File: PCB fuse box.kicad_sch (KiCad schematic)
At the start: 22 parts, among them J1 6570XX230201_657012230201, J2 6570XX230201_657012230201, J3 449140201, J4 449140201, K1 AZ2150-1A-12DEF, K2 AZ2150-1A-12DEF

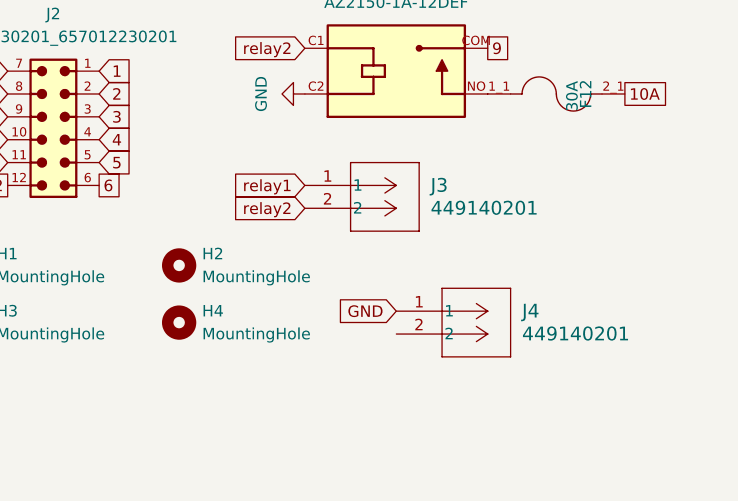
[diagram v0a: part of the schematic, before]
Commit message: fix smth
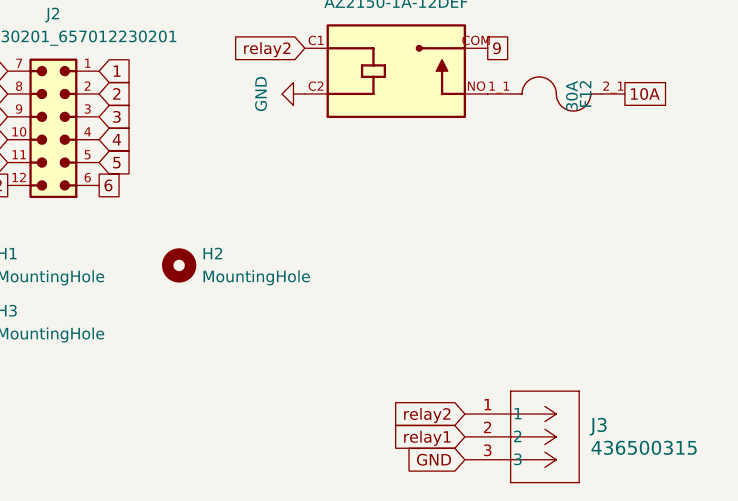
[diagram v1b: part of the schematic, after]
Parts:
- removed H4: MountingHole, MountingHole:MountingHole_2.2mm_M2_Pad, symbol Mechanical:MountingHole
- removed J3, J4: 449140201, fuse-relay_NewFootprints:CONN_SD-44914-002_02_MOL, symbol New_Library:449140201
- added J3: 436500315, MOLEX 436500315:CONN_SD-43650-006_03_MOL, symbol MOLEX 436500315:436500315
- F1, F10, F11, F12, F2, F3, F4, F5, F6, F7, F8, F9: footprint fuse-relay_NewFootprints:FUSE_3557-2 -> 3557:CONN_3557-2_KEY
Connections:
- net GND: now also J3.3
- net relay1: now also J3.2
- net relay2: now also J3.1
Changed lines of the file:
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@@
 	(global_label "relay1"
 		(shape input)
-		(at 104.14 77.47 180)
+		(at 121.92 105.41 180)
 		(fields_autoplaced yes)
 		(effects
@@
 		)
 		(property "Intersheetrefs" "${INTERSHEET_REFS}"
-			(at 95.2887 77.47 0)
+			(at 113.0687 105.41 0)
 			(hide yes)
 			(show_name no)
@@
 	(global_label "relay2"
 		(shape input)
-		(at 104.14 80.01 180)
+		(at 121.92 102.87 180)
 		(fields_autoplaced yes)
 		(effects
@@
 		)
 		(property "Intersheetrefs" "${INTERSHEET_REFS}"
-			(at 95.2887 80.01 0)
+			(at 113.0687 102.87 0)
 			(hide yes)
 			(show_name no)
@@
 	(global_label "GND"
 		(shape input)
-		(at 114.3 91.44 180)
+		(at 121.92 107.95 180)
 		(fields_autoplaced yes)
 		(effects
@@
 		)
 		(property "Intersheetrefs" "${INTERSHEET_REFS}"
-			(at 107.4443 91.44 0)
+			(at 115.0643 107.95 0)
 			(hide yes)
 			(show_name no)
@@
 	)
 	(symbol
+		(lib_id "MOLEX 436500315:436500315")
+		(at 121.92 102.87 0)
+		(unit 1)
+		(body_style 1)
+		(exclude_from_sim no)
+		(in_bom yes)
+		(on_board yes)
+		(in_pos_files yes)
+		(dnp no)
+		(fields_autoplaced yes)
+		(property "Reference" "J3"
+			(at 135.89 104.1399 0)
+			(show_name no)
+			(do_not_autoplace no)
+			(effects
+				(font
+					(size 1.524 1.524)
+				)
+				(justify left)
+			)
+		)
+		(property "Value" "436500315"
+			(at 135.89 106.6799 0)
+			(show_name no)
+			(do_not_autoplace no)
+			(effects
+				(font
+					(size 1.524 1.524)
+				)
+				(justify left)
+			)
+		)
+		(property "Footprint" "MOLEX 436500315:CONN_SD-43650-006_03_MOL"
+			(at 121.92 102.87 0)
+			(hide yes)
+			(show_name no)
+			(do_not_autoplace no)
+			(effects
+				(font
+					(size 1.27 1.27)
+					(italic yes)
+				)
+			)
+		)
+		(property "Datasheet" "https://www.molex.com/en-us/products/part-detail-pdf/436500315?display=pdf"
+			(at 121.92 102.87 0)
+			(hide yes)
+			(show_name no)
+			(do_not_autoplace no)
+			(effects
+				(font
+					(size 1.27 1.27)
+					(italic yes)
+				)
+			)
+		)
+		(property "Description" ""
+			(at 121.92 102.87 0)
+			(hide yes)
+			(show_name no)
+			(do_not_autoplace no)
+			(effects
+				(font
+					(size 1.27 1.27)
+				)
+			)
+		)
+		(pin "3"
+		)
+		(pin "1"
+		)
+		(pin "2"
+		)
+		(instances
+			(project "PCB fuse box"
+				(path "/edb1809c-767d-4732-82a5-e09154bd7612"
+					(reference "J3")
+					(unit 1)
+				)
+			)
+		)
+	)
+	(symbol
 		(lib_id "New_Library:3557-2")
 		(at 25.4 68.58 270)
@@
 			)
 		)
-		(property "Footprint" "fuse-relay_NewFootprints:FUSE_3557-2"
+		(property "Footprint" "3557:CONN_3557-2_KEY"
 			(at 25.4 68.58 0)
 			(hide yes)
@@
 			)
 		)
-		(property "Footprint" "fuse-relay_NewFootprints:FUSE_3557-2"
+		(property "Footprint" "3557:CONN_3557-2_KEY"
 			(at 35.56 41.91 0)
 			(hide yes)
@@
 			)
 		)
-		(property "Footprint" "fuse-relay_NewFootprints:FUSE_3557-2"
+		(property "Footprint" "3557:CONN_3557-2_KEY"
 			(at 55.88 68.58 0)
 			(hide yes)
@@
 	)
 	(symbol
-		(lib_id "Mechanical:MountingHole")
-		(at 90.17 92.71 0)
-		(unit 1)
-		(body_style 1)
-		(exclude_from_sim no)
-		(in_bom no)
-		(on_board yes)
-		(in_pos_files yes)
-		(dnp no)
-		(fields_autoplaced yes)
-		(property "Reference" "H4"
-			(at 92.71 91.4399 0)
-			(show_name no)
-			(do_not_autoplace no)
-			(effects
-				(font
-					(size 1.27 1.27)
-				)
-				(justify left)
-			)
-		)
-		(property "Value" "MountingHole"
-			(at 92.71 93.9799 0)
-			(show_name no)
-			(do_not_autoplace no)
-			(effects
-				(font
-					(size 1.27 1.27)
-				)
-				(justify left)
-			)
-		)
-		(property "Footprint" "MountingHole:MountingHole_2.2mm_M2_Pad"
-			(at 90.17 92.71 0)
-			(hide yes)
-			(show_name no)
-			(do_not_autoplace no)
-			(effects
-				(font
-					(size 1.27 1.27)
-				)
-			)
-		)
-		(property "Datasheet" ""
-			(at 90.17 92.71 0)
-			(hide yes)
-			(show_name no)
-			(do_not_autoplace no)
-			(effects
-				(font
-					(size 1.27 1.27)
-				)
-			)
-		)
-		(property "Description" "Mounting Hole without connection"
-			(at 90.17 92.71 0)
-			(hide yes)
-			(show_name no)
-			(do_not_autoplace no)
-			(effects
-				(font
-					(size 1.27 1.27)
-				)
-			)
-		)
-		(instances
-			(project "PCB fuse box"
-				(path "/edb1809c-767d-4732-82a5-e09154bd7612"
-					(reference "H4")
-					(unit 1)
-				)
-			)
-		)
-	)
-	(symbol
 		(lib_id "New_Library:3557-2")
 		(at 36.83 93.98 270)
@@
 			)
 		)
-		(property "Footprint" "fuse-relay_NewFootprints:FUSE_3557-2"
+		(property "Footprint" "3557:CONN_3557-2_KEY"
 			(at 36.83 93.98 0)
 			(hide yes)
@@
 			)
 		)
-		(property "Footprint" "fuse-relay_NewFootprints:FUSE_3557-2"
+		(property "Footprint" "3557:CONN_3557-2_KEY"
 			(at 132.08 41.91 0)
 			(hide yes)
@@
 			)
 		)
-		(property "Footprint" "fuse-relay_NewFootprints:FUSE_3557-2"
+		(property "Footprint" "3557:CONN_3557-2_KEY"
 			(at 35.56 68.58 0)
 			(hide yes)
@@
 	)
 	(symbol
-		(lib_id "New_Library:449140201")
-		(at 114.3 91.44 0)
-		(unit 1)
-		(body_style 1)
-		(exclude_from_sim no)
-		(in_bom yes)
-		(on_board yes)
-		(in_pos_files yes)
-		(dnp no)
-		(fields_autoplaced yes)
-		(property "Reference" "J4"
-			(at 128.27 91.4399 0)
-			(show_name no)
-			(do_not_autoplace no)
-			(effects
-				(font
-					(size 1.524 1.524)
-				)
-				(justify left)
-			)
-		)
-		(property "Value" "449140201"
-			(at 128.27 93.9799 0)
-			(show_name no)
-			(do_not_autoplace no)
-			(effects
-				(font
-					(size 1.524 1.524)
-				)
-				(justify left)
-			)
-		)
-		(property "Footprint" "fuse-relay_NewFootprints:CONN_SD-44914-002_02_MOL"
-			(at 114.3 91.44 0)
-			(hide yes)
-			(show_name no)
-			(do_not_autoplace no)
-			(effects
-				(font
-					(size 1.27 1.27)
-					(italic yes)
-				)
-			)
-		)
-		(property "Datasheet" "https://www.molex.com/en-us/products/part-detail-pdf/449140201?display=pdf"
-			(at 114.3 91.44 0)
-			(hide yes)
-			(show_name no)
-			(do_not_autoplace no)
-			(effects
-				(font
-					(size 1.27 1.27)
-					(italic yes)
-				)
-			)
-		)
-		(property "Description" ""
-			(at 114.3 91.44 0)
-			(hide yes)
-			(show_name no)
-			(do_not_autoplace no)
-			(effects
-				(font
-					(size 1.27 1.27)
-				)
-			)
-		)
-		(pin "1"
-		)
-		(pin "2"
-		)
-		(instances
-			(project "PCB fuse box"
-				(path "/edb1809c-767d-4732-82a5-e09154bd7612"
-					(reference "J4")
-					(unit 1)
-				)
-			)
-		)
-	)
-	(symbol
 		(lib_id "New_Library:3557-2")
 		(at 45.72 68.58 270)
@@
 			)
 		)
-		(property "Footprint" "fuse-relay_NewFootprints:FUSE_3557-2"
+		(property "Footprint" "3557:CONN_3557-2_KEY"
 			(at 45.72 68.58 0)
 			(hide yes)
@@
 	)
 	(symbol
-		(lib_id "New_Library:449140201")
-		(at 104.14 77.47 0)
-		(unit 1)
-		(body_style 1)
-		(exclude_from_sim no)
-		(in_bom yes)
-		(on_board yes)
-		(in_pos_files yes)
-		(dnp no)
-		(fields_autoplaced yes)
-		(property "Reference" "J3"
-			(at 118.11 77.4699 0)
-			(show_name no)
-			(do_not_autoplace no)
-			(effects
-				(font
-					(size 1.524 1.524)
-				)
-				(justify left)
-			)
-		)
-		(property "Value" "449140201"
-			(at 118.11 80.0099 0)
-			(show_name no)
-			(do_not_autoplace no)
-			(effects
-				(font
-					(size 1.524 1.524)
-				)
-				(justify left)
-			)
-		)
-		(property "Footprint" "fuse-relay_NewFootprints:CONN_SD-44914-002_02_MOL"
-			(at 104.14 77.47 0)
-			(hide yes)
-			(show_name no)
-			(do_not_autoplace no)
-			(effects
-				(font
-					(size 1.27 1.27)
-					(italic yes)
-				)
-			)
-		)
-		(property "Datasheet" "https://www.molex.com/en-us/products/part-detail-pdf/449140201?display=pdf"
-			(at 104.14 77.47 0)
-			(hide yes)
-			(show_name no)
-			(do_not_autoplace no)
-			(effects
-				(font
-					(size 1.27 1.27)
-					(italic yes)
-				)
-			)
-		)
-		(property "Description" ""
-			(at 104.14 77.47 0)
-			(hide yes)
-			(show_name no)
-			(do_not_autoplace no)
-			(effects
-				(font
-					(size 1.27 1.27)
-				)
-			)
-		)
-		(pin "1"
-		)
-		(pin "2"
-		)
-		(instances
-			(project "PCB fuse box"
-				(path "/edb1809c-767d-4732-82a5-e09154bd7612"
-					(reference "J3")
-					(unit 1)
-				)
-			)
-		)
-	)
-	(symbol
 		(lib_id "New_Library:3557-2")
 		(at 55.88 41.91 270)
@@
 			)
 		)
-		(property "Footprint" "fuse-relay_NewFootprints:FUSE_3557-2"
+		(property "Footprint" "3557:CONN_3557-2_KEY"
 			(at 55.88 41.91 0)
 			(hide yes)
@@
 			)
 		)
-		(property "Footprint" "fuse-relay_NewFootprints:FUSE_3557-2"
+		(property "Footprint" "3557:CONN_3557-2_KEY"
 			(at 45.72 41.91 0)
 			(hide yes)
@@
 			)
 		)
-		(property "Footprint" "fuse-relay_NewFootprints:FUSE_3557-2"
+		(property "Footprint" "3557:CONN_3557-2_KEY"
 			(at 46.99 93.98 0)
 			(hide yes)
@@
 			)
 		)
-		(property "Footprint" "fuse-relay_NewFootprints:FUSE_3557-2"
+		(property "Footprint" "3557:CONN_3557-2_KEY"
 			(at 132.08 67.31 0)
 			(hide yes)
@@
 			)
 		)
-		(property "Footprint" "fuse-relay_NewFootprints:FUSE_3557-2"
+		(property "Footprint" "3557:CONN_3557-2_KEY"
 			(at 25.4 41.91 0)
 			(hide yes)
